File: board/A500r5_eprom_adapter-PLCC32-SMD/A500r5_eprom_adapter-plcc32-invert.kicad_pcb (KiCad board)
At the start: 2 copper layers, 40.6 x 54.6 mm, 12 parts, among them J2 A18 Selector, J3 A19 Selector, J4 A17 Selector, U1 27C400-A500, U2 27C080-L, U3 27C080-L

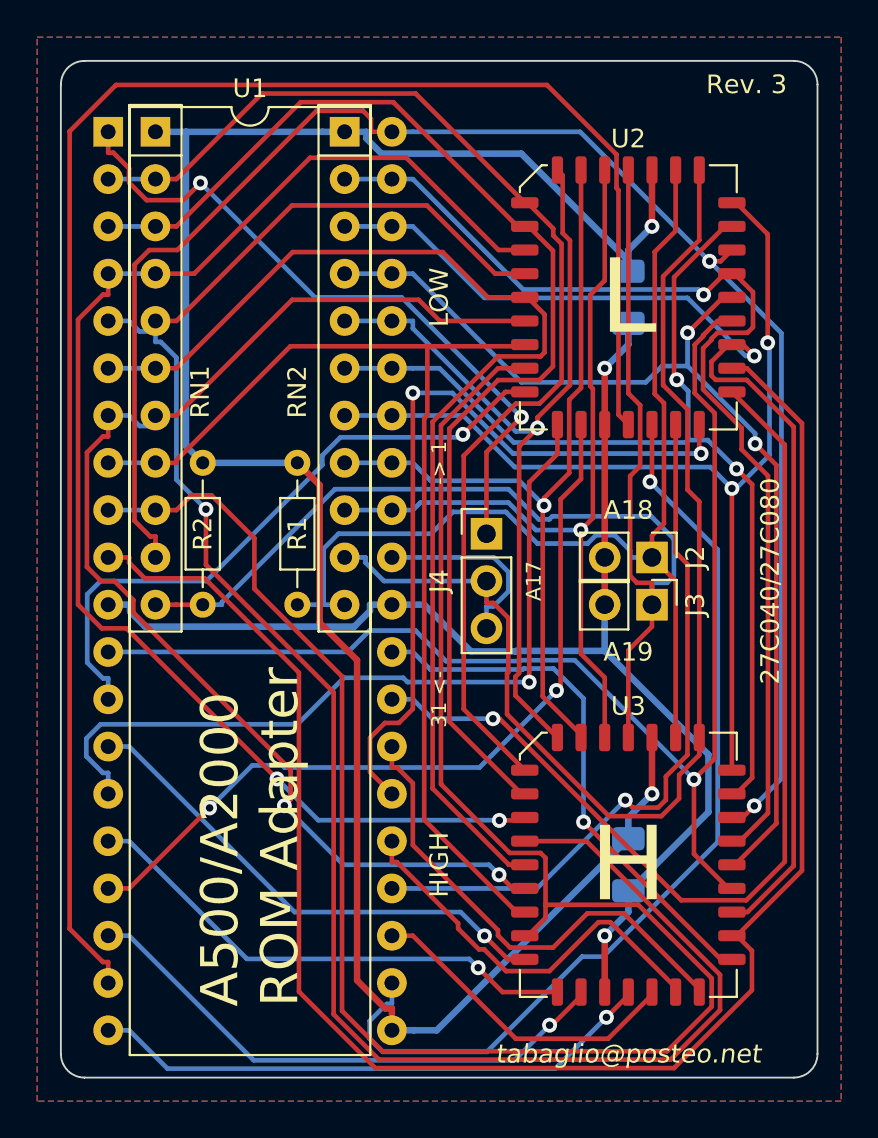
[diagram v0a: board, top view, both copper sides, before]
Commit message: Create an SMD rev 4
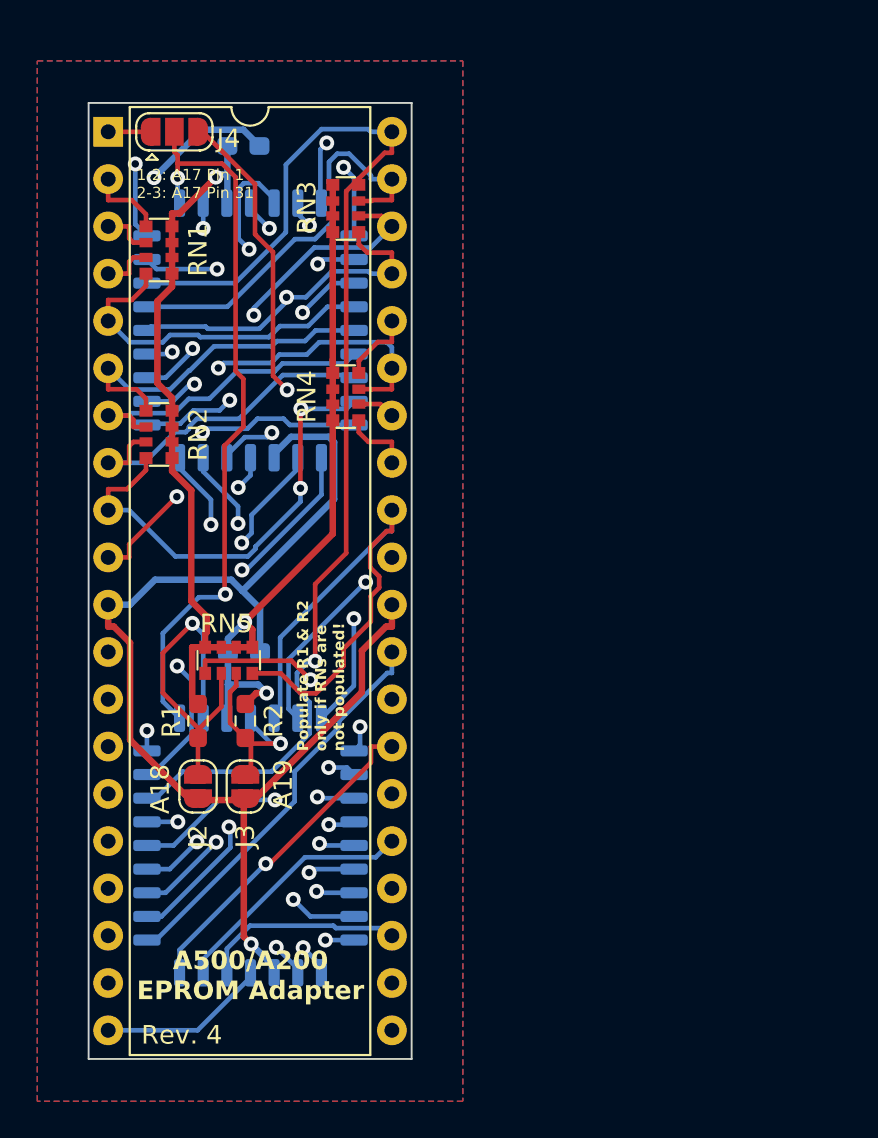
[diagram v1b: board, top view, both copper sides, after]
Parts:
- added RN3: 4.7K, Resistor_SMD:R_Array_Convex_4x0612, F.Cu at (123.3, 79.0)
- added RN4: 4.7K, Resistor_SMD:R_Array_Convex_4x0612, F.Cu at (123.3, 89.2)
- added RN5: 4.7K, Resistor_SMD:R_Array_Convex_4x0612, F.Cu at (117.0, 103.3)
- C1, C2: footprint Capacitor_SMD:C_1206_3216Metric -> Capacitor_SMD:C_0603_1608Metric_Pad1.08x0.95mm_HandSolder
- J2, J3: footprint Connector_PinHeader_2.54mm:PinHeader_1x02_P2.54mm_Vertical -> Jumper:SolderJumper-2_P1.3mm_Open_RoundedPad1.0x1.5mm
- J4: footprint Connector_PinHeader_2.54mm:PinHeader_1x03_P2.54mm_Vertical -> Jumper:SolderJumper-3_P1.3mm_Open_RoundedPad1.0x1.5mm
- R1, R2: value 4k7 -> 4.7K; footprint Resistor_THT:R_Axial_DIN0204_L3.6mm_D1.6mm_P7.62mm_Horizontal -> Resistor_SMD:R_0603_1608Metric_Pad0.98x0.95mm_HandSolder
- RN1, RN2: value 4k7 -> 4.7K; footprint Resistor_THT:R_Array_SIP11 -> Resistor_SMD:R_Array_Convex_4x0612
- U2, U3: moved to B.Cu
- moved J4 27.3 mm to (114.0, 74.9)
- moved J2 27.3 mm to (115.3, 110.1)
- moved J3 23.9 mm to (117.9, 110.1)
- moved C1 23.6 mm to (117.8, 102.9), turned to 0 degrees
- moved C2 22.2 mm to (117.8, 75.7), turned to 0 degrees
- moved U2 20.4 mm to (118.1, 85.6), turned to 180 degrees
- moved U3 20.3 mm to (118.1, 113.3), turned to 180 degrees
- moved RN2 19.1 mm to (113.2, 91.2), turned to 180 degrees
- moved R1 14.9 mm to (115.3, 106.6), turned to 90 degrees
- moved R2 14.1 mm to (117.9, 106.6), turned to 90 degrees
- moved RN1 6.35 mm to (113.2, 81.3), turned to 180 degrees
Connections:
- net /~CE renamed /~{CE}
- net /~OE renamed /~{OE}
- R1 pad 1: VCC -> /A18
- R1 pad 2: /A18 -> VCC
- R2 pad 1: VCC -> /A19
- R2 pad 2: /A19 -> VCC
- RN1 pad 2: /A7 -> VCC
- RN1 pad 3: /A6 -> VCC
- RN1 pad 4: /A5 -> VCC
- RN1 pad 5: /A4 -> /A7
- RN1 pad 6: /A3 -> /A6
- RN1 pad 7: /A2 -> /A5
- RN1 pad 8: /A1 -> /A4
- RN2 pad 2: /A9 -> VCC
- RN2 pad 3: /A10 -> VCC
- RN2 pad 4: /A11 -> VCC
- RN2 pad 5: /A12 -> /A3
- RN2 pad 6: /A13 -> /A2
- RN2 pad 7: /A14 -> /A1
- RN2 pad 8: /A15 -> /A0
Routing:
- net /D3-L: track 93.5 -> 33.4 mm, vias 0 -> 1
- net /~{CE}: track 95.4 -> 39.3 mm, vias 0 -> 3
- net /A4: track 106.3 -> 52.3 mm
- net /A0: track 107.3 -> 53.7 mm, vias 0 -> 3
- net /SOCK_P1: track 37.5 -> 2.26 mm, vias 2 -> 0
- net /~{OE}: track 68.9 -> 34.7 mm, vias 1 -> 2
- net /D7-L: track 52.8 -> 24.8 mm
- net /A5: track 74.5 -> 47.1 mm
- net /A19: track 68.7 -> 41.5 mm, vias 0 -> 2
- net GND: track 70.2 -> 96.5 mm
- net /A8: track 88.8 -> 64.4 mm, vias 2 -> 1
- net /D3-H: track 30.6 -> 9.07 mm, vias 1 -> 0
- net /D1-L: track 43.3 -> 23.4 mm
- net /A2: track 67.7 -> 48.8 mm, vias 2 -> 1
- net /D2-H: track 29.8 -> 11.4 mm
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- added copper zone on In1.Cu, net GND
- added copper zone on In2.Cu, net GND
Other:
- board size 40.6 x 54.6 mm -> 17.4 x 51.4 mm
- copper layers 2 -> 4
- net class Default removed
- net class POWER removed
- board text added: "1-2: A17 Pin 1 2-3: A17 Pin 31"
- board text added: "A500/A200 EPROM Adapter"
- board text added: "Populate R1 & R2 only if RNs are not populated!"
- board text added: "Rev. 4"
- board text removed: "-> 1"
- board text removed: "27C040/27C080"
- board text removed: "31 <-"
- board text removed: "A17"
- board text removed: "A500/A2000 ROM Adapter"
- board text removed: "HIGH"
- board text removed: "LOW"
- board text removed: "Rev. 3"
- board text removed: "tabaglio@posteo.net"
